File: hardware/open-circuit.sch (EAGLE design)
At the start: 75 parts, among them IC1 PIC16F1825SO14, IC2 74HC595D, IC3 MCP4728_QUAD_DAC, IC4 LM324D, IC5 REG1117, IC6 LM27675M5_CHARGEPUMP

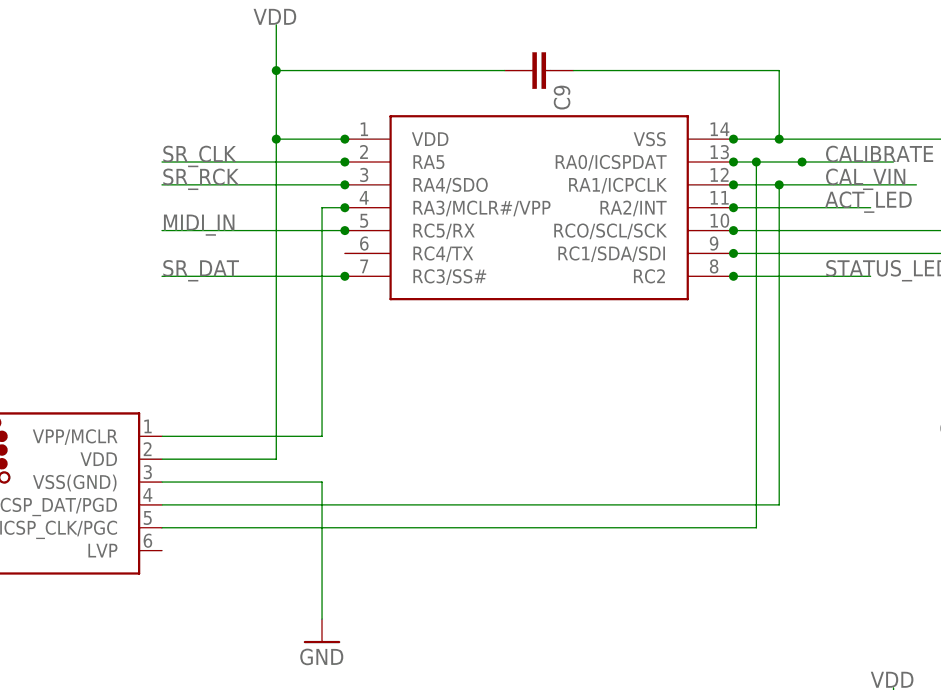
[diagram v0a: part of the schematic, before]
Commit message: initial test of pcb
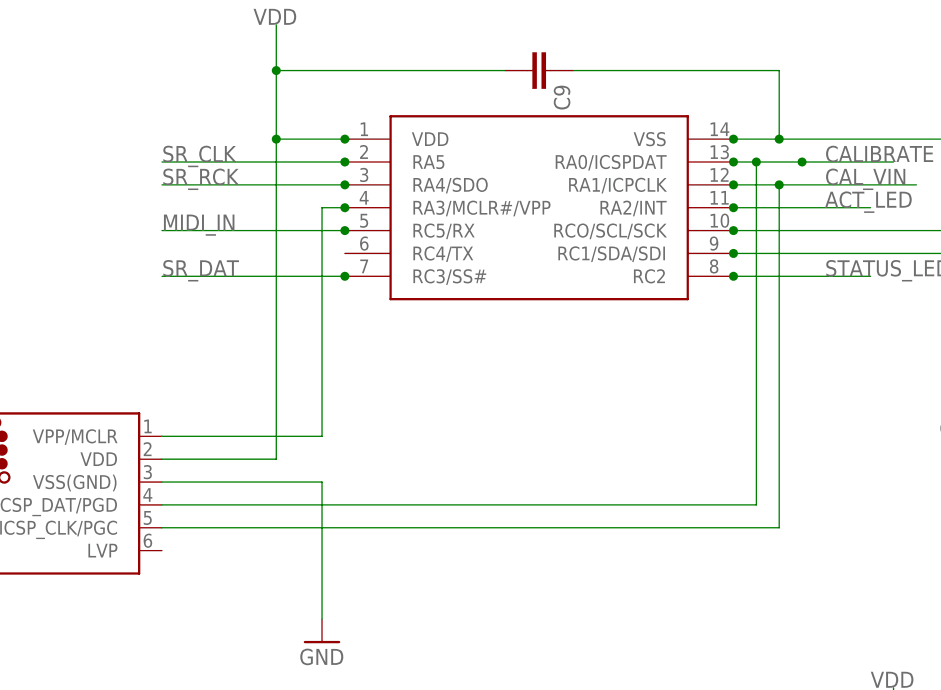
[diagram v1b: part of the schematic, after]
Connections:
- net CALIBRATE: now also ISCP.ICSP_DAT/PGD; no longer ISCP.ICSP_CLK/PGC
- net CAL_VIN: now also ISCP.ICSP_CLK/PGC; no longer ISCP.ICSP_DAT/PGD
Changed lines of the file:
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@@
 </segment>
 <segment>
-<pinref part="ISCP" gate="G$1" pin="ICSP_DAT/PGD"/>
-<wire x1="-111.76" y1="48.26" x2="-43.18" y2="48.26" width="0.1524" layer="91"/>
-<wire x1="-43.18" y1="48.26" x2="-43.18" y2="83.82" width="0.1524" layer="91"/>
+<wire x1="-43.18" y1="45.72" x2="-43.18" y2="83.82" width="0.1524" layer="91"/>
 <label x="-38.1" y="83.82" size="1.778" layer="95"/>
 <junction x="-43.18" y="83.82"/>
@@
 <pinref part="IC1" gate="G$1" pin="RA1/ICPCLK"/>
 <junction x="-48.26" y="83.82"/>
+<pinref part="ISCP" gate="G$1" pin="ICSP_CLK/PGC"/>
+<wire x1="-111.76" y1="45.72" x2="-43.18" y2="45.72" width="0.1524" layer="91"/>
 </segment>
 </net>
@@
 </segment>
 <segment>
-<pinref part="ISCP" gate="G$1" pin="ICSP_CLK/PGC"/>
-<wire x1="-111.76" y1="45.72" x2="-45.72" y2="45.72" width="0.1524" layer="91"/>
-<wire x1="-45.72" y1="45.72" x2="-45.72" y2="86.36" width="0.1524" layer="91"/>
+<wire x1="-45.72" y1="48.26" x2="-45.72" y2="86.36" width="0.1524" layer="91"/>
 <wire x1="-45.72" y1="86.36" x2="-40.64" y2="86.36" width="0.1524" layer="91"/>
 <label x="-38.1" y="86.36" size="1.778" layer="95"/>
@@
 <junction x="-45.72" y="86.36"/>
 <junction x="-48.26" y="86.36"/>
+<pinref part="ISCP" gate="G$1" pin="ICSP_DAT/PGD"/>
+<wire x1="-111.76" y1="48.26" x2="-45.72" y2="48.26" width="0.1524" layer="91"/>
 </segment>
 </net>

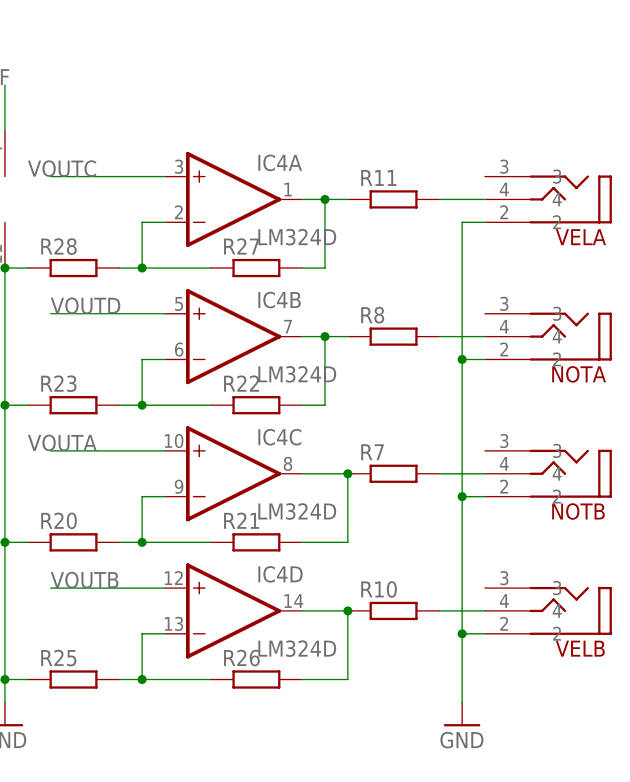
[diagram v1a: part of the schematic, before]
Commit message: updates
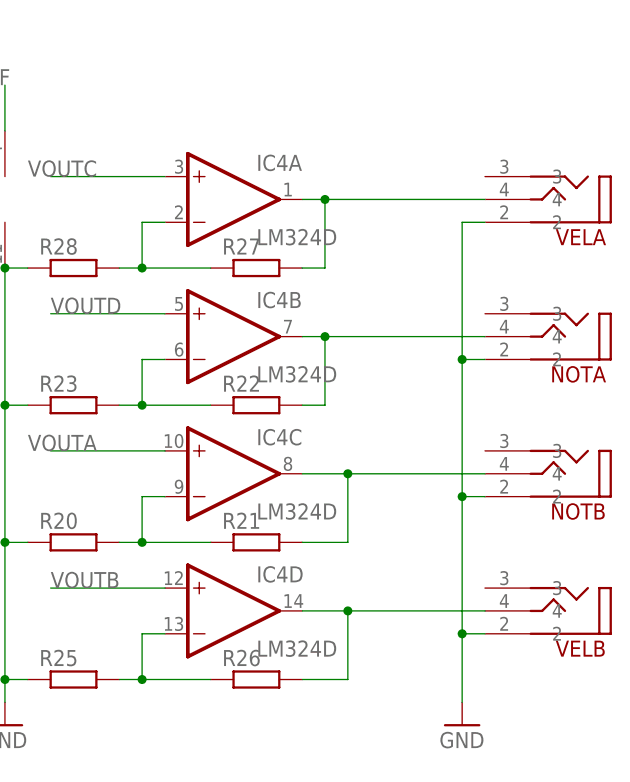
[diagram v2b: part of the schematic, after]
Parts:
- removed R10, R11, R7, R8: (no value), rcl:R-EU_R0805
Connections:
- removed net N$29: R11.2, VELA.4
- removed net N$30: NOTA.4, R8.2
- removed net N$31: NOTB.4, R7.2
- removed net N$32: R10.2, VELB.4
- net N$2: now also VELA.4; no longer R11.1
- net N$3: now also NOTA.4; no longer R8.1
- net N$4: now also NOTB.4; no longer R7.1
- net N$5: now also VELB.4; no longer R10.1
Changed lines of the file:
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@@
 <part name="GND12" library="supply1" deviceset="GND" device=""/>
 <part name="IC4" library="linear" deviceset="LM324" device="D"/>
-<part name="R8" library="rcl" deviceset="R-EU_" device="R0805"/>
-<part name="R11" library="rcl" deviceset="R-EU_" device="R0805"/>
-<part name="R7" library="rcl" deviceset="R-EU_" device="R0805"/>
-<part name="R10" library="rcl" deviceset="R-EU_" device="R0805"/>
 <part name="R27" library="rcl" deviceset="R-EU_" device="R0805"/>
 <part name="R22" library="rcl" deviceset="R-EU_" device="R0805"/>
@@
 <instance part="IC4" gate="C" x="114.3" y="83.82"/>
 <instance part="IC4" gate="D" x="114.3" y="68.58"/>
-<instance part="R8" gate="G$1" x="132.08" y="99.06"/>
-<instance part="R11" gate="G$1" x="132.08" y="114.3"/>
-<instance part="R7" gate="G$1" x="132.08" y="83.82"/>
-<instance part="R10" gate="G$1" x="132.08" y="68.58"/>
 <instance part="R27" gate="G$1" x="116.84" y="106.68"/>
 <instance part="R22" gate="G$1" x="116.84" y="91.44"/>
@@
 <wire x1="121.92" y1="106.68" x2="124.46" y2="106.68" width="0.1524" layer="91"/>
 <pinref part="IC4" gate="A" pin="OUT"/>
-<pinref part="R11" gate="G$1" pin="1"/>
 <wire x1="121.92" y1="114.3" x2="124.46" y2="114.3" width="0.1524" layer="91"/>
-<wire x1="124.46" y1="114.3" x2="127" y2="114.3" width="0.1524" layer="91"/>
 <wire x1="124.46" y1="106.68" x2="124.46" y2="114.3" width="0.1524" layer="91"/>
 <junction x="124.46" y="114.3"/>
+<pinref part="VELA" gate="G$1" pin="4"/>
+<wire x1="124.46" y1="114.3" x2="142.24" y2="114.3" width="0.1524" layer="91"/>
 </segment>
 </net>
@@
 <wire x1="121.92" y1="91.44" x2="124.46" y2="91.44" width="0.1524" layer="91"/>
 <pinref part="IC4" gate="B" pin="OUT"/>
-<pinref part="R8" gate="G$1" pin="1"/>
 <wire x1="121.92" y1="99.06" x2="124.46" y2="99.06" width="0.1524" layer="91"/>
-<wire x1="124.46" y1="99.06" x2="127" y2="99.06" width="0.1524" layer="91"/>
 <wire x1="124.46" y1="91.44" x2="124.46" y2="99.06" width="0.1524" layer="91"/>
 <junction x="124.46" y="99.06"/>
+<pinref part="NOTA" gate="G$1" pin="4"/>
+<wire x1="124.46" y1="99.06" x2="142.24" y2="99.06" width="0.1524" layer="91"/>
 </segment>
 </net>
@@
 <segment>
 <pinref part="IC4" gate="C" pin="OUT"/>
-<pinref part="R7" gate="G$1" pin="1"/>
 <wire x1="121.92" y1="83.82" x2="127" y2="83.82" width="0.1524" layer="91"/>
 <pinref part="R21" gate="G$1" pin="2"/>
 <wire x1="121.92" y1="76.2" x2="127" y2="76.2" width="0.1524" layer="91"/>
 <wire x1="127" y1="76.2" x2="127" y2="83.82" width="0.1524" layer="91"/>
+<pinref part="NOTB" gate="G$1" pin="4"/>
+<wire x1="127" y1="83.82" x2="142.24" y2="83.82" width="0.1524" layer="91"/>
 <junction x="127" y="83.82"/>
 </segment>
@@
 <segment>
 <pinref part="IC4" gate="D" pin="OUT"/>
-<pinref part="R10" gate="G$1" pin="1"/>
 <wire x1="121.92" y1="68.58" x2="127" y2="68.58" width="0.1524" layer="91"/>
 <pinref part="R26" gate="G$1" pin="2"/>
 <wire x1="121.92" y1="60.96" x2="127" y2="60.96" width="0.1524" layer="91"/>
 <wire x1="127" y1="60.96" x2="127" y2="68.58" width="0.1524" layer="91"/>
+<pinref part="VELB" gate="G$1" pin="4"/>
+<wire x1="127" y1="68.58" x2="142.24" y2="68.58" width="0.1524" layer="91"/>
 <junction x="127" y="68.58"/>
 </segment>
@@
 <wire x1="45.72" y1="78.74" x2="60.96" y2="78.74" width="0.1524" layer="91"/>
 <label x="58.42" y="78.74" size="1.778" layer="95"/>
-</segment>
-</net>
-<net name="N$31" class="0">
-<segment>
-<pinref part="R7" gate="G$1" pin="2"/>
-<pinref part="NOTB" gate="G$1" pin="4"/>
-<wire x1="137.16" y1="83.82" x2="142.24" y2="83.82" width="0.1524" layer="91"/>
-</segment>
-</net>
-<net name="N$32" class="0">
-<segment>
-<pinref part="R10" gate="G$1" pin="2"/>
-<pinref part="VELB" gate="G$1" pin="4"/>
-<wire x1="137.16" y1="68.58" x2="142.24" y2="68.58" width="0.1524" layer="91"/>
 </segment>
 </net>
@@
 </segment>
 </net>
-<net name="N$29" class="0">
-<segment>
-<pinref part="R11" gate="G$1" pin="2"/>
-<pinref part="VELA" gate="G$1" pin="4"/>
-<wire x1="137.16" y1="114.3" x2="142.24" y2="114.3" width="0.1524" layer="91"/>
-</segment>
-</net>
-<net name="N$30" class="0">
-<segment>
-<pinref part="R8" gate="G$1" pin="2"/>
-<pinref part="NOTA" gate="G$1" pin="4"/>
-<wire x1="137.16" y1="99.06" x2="142.24" y2="99.06" width="0.1524" layer="91"/>
-</segment>
-</net>
